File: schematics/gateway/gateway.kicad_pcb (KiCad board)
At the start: 2 copper layers, 152 x 101 mm, 10 parts, among them J1 Power, SW1 SW_Push

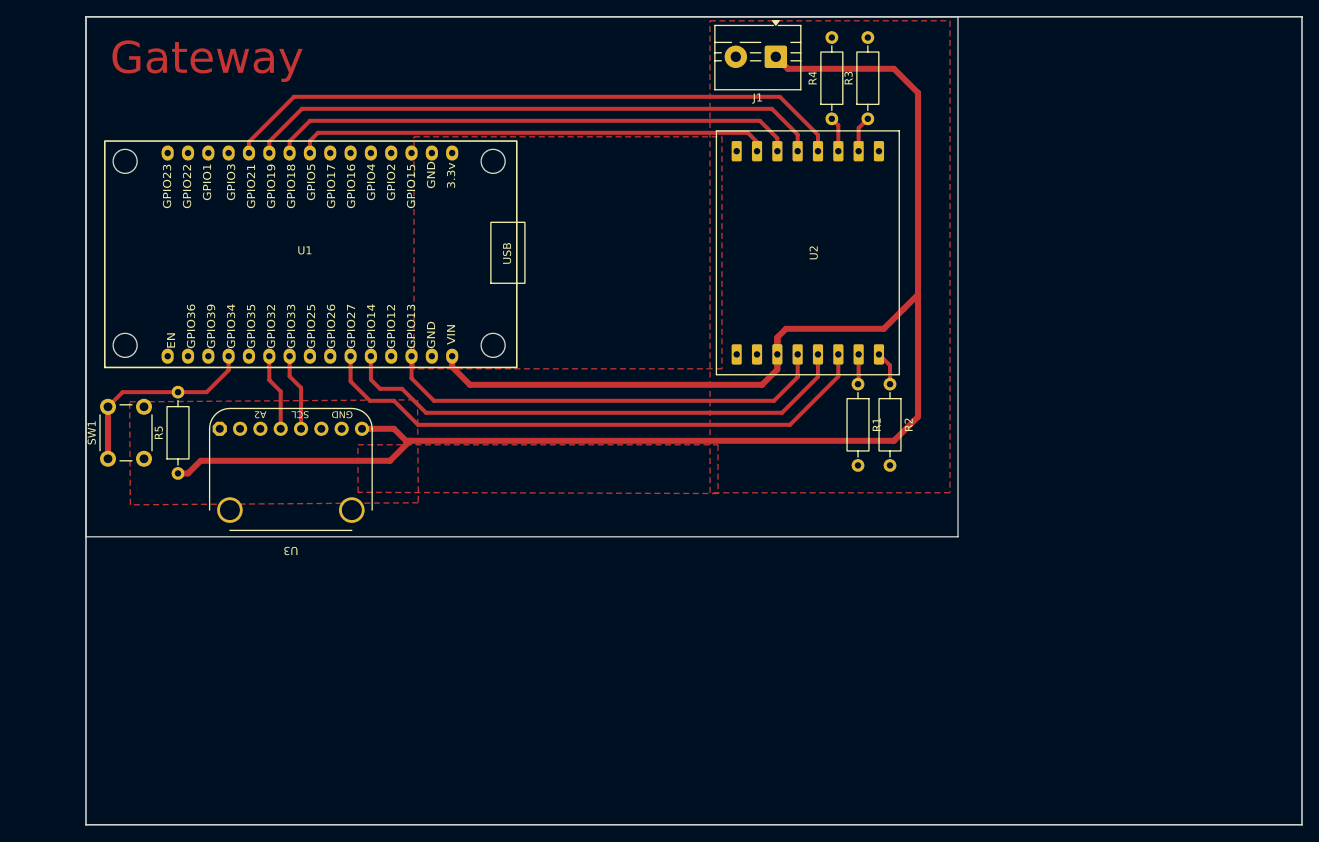
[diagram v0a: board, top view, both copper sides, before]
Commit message: updated pcb and schematics
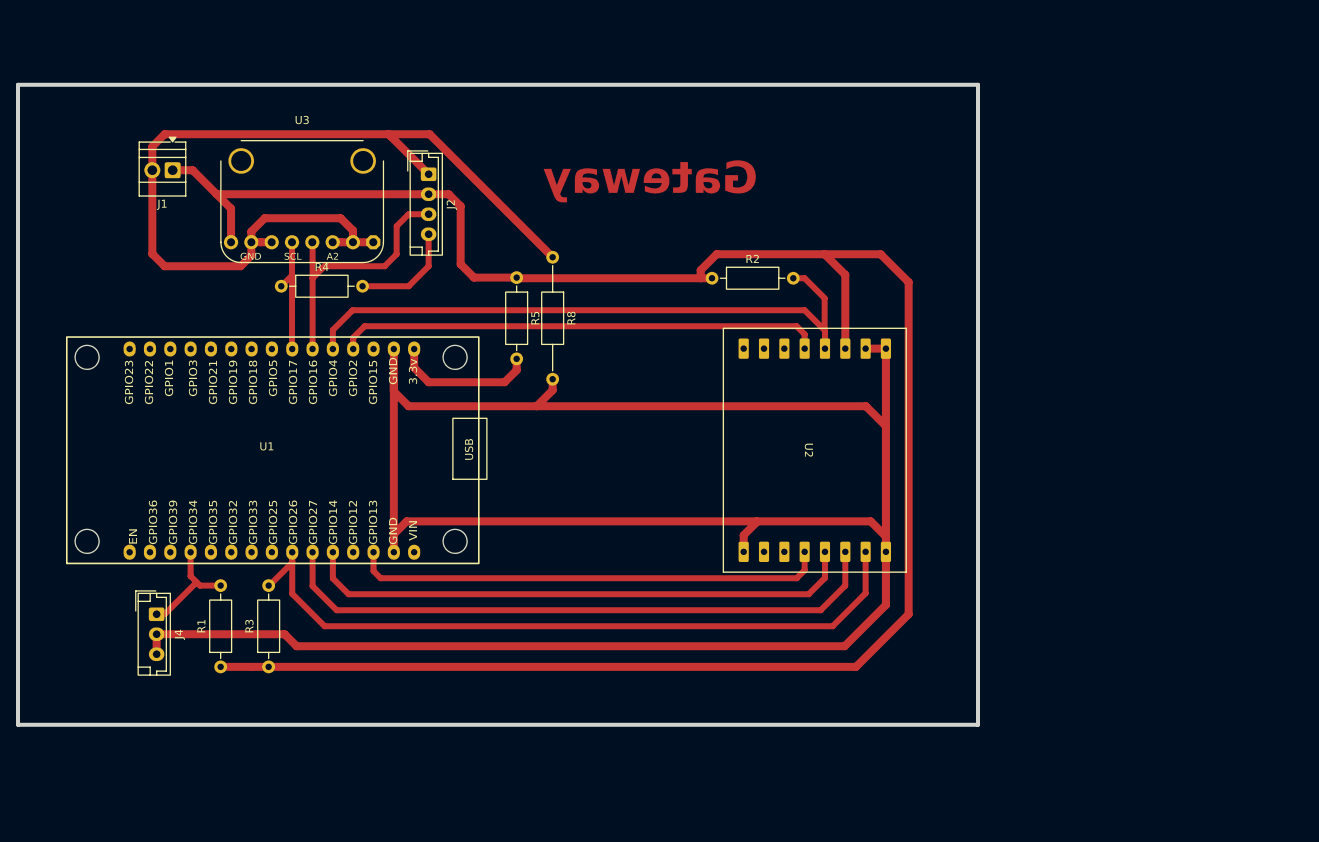
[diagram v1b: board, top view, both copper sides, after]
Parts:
- removed SW1: SW_Push, Button_Switch_THT:SW_PUSH_6mm
- added J2: PN532_Port, Connector_JST:JST_EH_B4B-EH-A_1x04_P2.50mm_Vertical, F.Cu at (81.3, 49.7)
- added J4: Button_Port, Connector_JST:JST_EH_B3B-EH-A_1x03_P2.50mm_Vertical, F.Cu at (47.3, 104.7)
- added R8: 0, Resistor_THT:R_Axial_DIN0207_L6.3mm_D2.5mm_P15.24mm_Horizontal, F.Cu at (96.8, 60.1)
- J1: footprint TerminalBlock:TerminalBlock_MaiXu_MX126-5.0-02P_1x02_P5.00mm -> TerminalBlock:TerminalBlock_Xinya_XY308-2.54-2P_1x02_P2.54mm_Horizontal
- R4, R5: value 10k -> 0
- moved R3 101.5 mm to (61.3, 111.3)
- moved R1 87.2 mm to (55.3, 111.3), turned to 90 degrees
- moved J1 76.7 mm to (49.3, 49.2)
- moved R4 71.9 mm to (62.9, 63.7), turned to 0 degrees
- moved R5 48.9 mm to (92.3, 62.6), turned to -90 degrees
- moved U3 35.1 mm to (65.5, 52.3), turned to 0 degrees
- moved R2 25.9 mm to (116.8, 62.7), turned to 0 degrees
- moved U1 25.0 mm to (62.5, 85.0)
- moved U2 24.7 mm to (128.3, 84.2), turned to -90 degrees
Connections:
- J1 pad 1: 3V3 -> +3V3
- R1 pad 1: Net-(U2-DIO2) -> +3V3
- R1 pad 2: GND -> /BTN_POLE
- R2 pad 1: Net-(U2-DIO3) -> +3V3
- R2 pad 2: GND -> /LORA_RST
- R3 pad 1: Net-(U2-DIO4) -> +3V3
- R3 pad 2: GND -> /LORA_NSS
- R4 pad 1: Net-(U2-DIO5) -> /I2C_SCL
- R4 pad 2: GND -> Net-(J2-Pin_4)
- R5 pad 1: 3V3 -> +3V3
- R5 pad 2: Net-(U1-GPIO34) -> Net-(U1-3.3v)
- U1 pad 1: 3V3 -> unconnected-(U1-VIN-Pad1)
- U1 pad 10: /FRAM_SDA -> unconnected-(U1-GPIO32-Pad10)
- U1 pad 12: Net-(U1-GPIO34) -> /BTN_POLE
- U1 pad 16: unconnected-(U1-3.3v-Pad16) -> Net-(U1-3.3v)
- U1 pad 17: GND -> GND2
- U1 pad 19: unconnected-(U1-GPIO2-Pad19) -> /LORA_DIO0
- U1 pad 2: GND -> GND2
- U1 pad 20: unconnected-(U1-GPIO4-Pad20) -> /LORA_RST
- U1 pad 21: unconnected-(U1-GPIO16-Pad21) -> /I2C_SDA
- U1 pad 22: unconnected-(U1-GPIO17-Pad22) -> /I2C_SCL
- U1 pad 23: /LoRa_NSS -> unconnected-(U1-GPIO5-Pad23)
- U1 pad 24: /LoRa_MOSI -> unconnected-(U1-GPIO18-Pad24)
- U1 pad 25: /LoRa_MISO -> unconnected-(U1-GPIO19-Pad25)
- U1 pad 26: /LoRa_SCK -> unconnected-(U1-GPIO21-Pad26)
- U1 pad 3: /LoRa_RST -> /LORA_SCK
- U1 pad 5: /LoRa_DIO0 -> /LORA_MISO
- U1 pad 6: /LoRa_DIO1 -> /LORA_MOSI
- U1 pad 7: unconnected-(U1-GPIO26-Pad7) -> /LORA_NSS
- U1 pad 9: /FRAM_SCL -> unconnected-(U1-GPIO33-Pad9)
- U2 pad 1: GND -> GND2
- U2 pad 10: /LoRa_NSS -> /LORA_NSS
- U2 pad 11: /LoRa_MOSI -> /LORA_MOSI
- U2 pad 12: /LoRa_MISO -> /LORA_MISO
- U2 pad 13: /LoRa_SCK -> /LORA_SCK
- U2 pad 2: 3V3 -> +3V3
- U2 pad 3: /LoRa_RST -> /LORA_RST
- U2 pad 4: /LoRa_DIO0 -> /LORA_DIO0
- U2 pad 5: /LoRa_DIO1 -> unconnected-(U2-DIO1-Pad5)
- U2 pad 6: Net-(U2-DIO2) -> unconnected-(U2-DIO2-Pad6)
- U2 pad 7: Net-(U2-DIO3) -> unconnected-(U2-DIO3-Pad7)
- U2 pad 8: Net-(U2-DIO4) -> unconnected-(U2-DIO4-Pad8)
- U2 pad 9: Net-(U2-DIO5) -> unconnected-(U2-DIO5-Pad9)
- U3 pad 4: /FRAM_SDA -> /I2C_SDA
- U3 pad 5: /FRAM_SCL -> /I2C_SCL
- U3 pad 8: 3V3 -> +3V3
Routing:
- net GND2: track 0.00 -> 292.5 mm
- net +3V3: track 0.00 -> 256.4 mm
- net 3V3: track 232.8 -> 0.00 mm
- net GND: track 0.00 -> 117.2 mm
- net /LORA_NSS: track 0.00 -> 91.0 mm
- net /LoRa_SCK: track 78.9 -> 0.00 mm
- net /LORA_MOSI: track 0.00 -> 77.6 mm
- net /LORA_RST: track 0.00 -> 77.2 mm
- net /LoRa_MISO: track 72.6 -> 0.00 mm
- net /LoRa_DIO1: track 71.6 -> 0.00 mm
- net /LORA_MISO: track 0.00 -> 69.7 mm
- net /LoRa_MOSI: track 66.0 -> 0.00 mm
- net /LoRa_DIO0: track 65.2 -> 0.00 mm
- net /LORA_DIO0: track 0.00 -> 60.7 mm
- net /LoRa_NSS: track 59.5 -> 0.00 mm
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- removed copper zone on F.Cu, net GND
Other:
- board size 152 x 101 mm -> 120 x 80 mm
